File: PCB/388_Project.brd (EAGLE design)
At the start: 88.6 x 79.1 mm, 37 parts, among them IC1 7824DT, U1 ATMEGA328P_TQFP

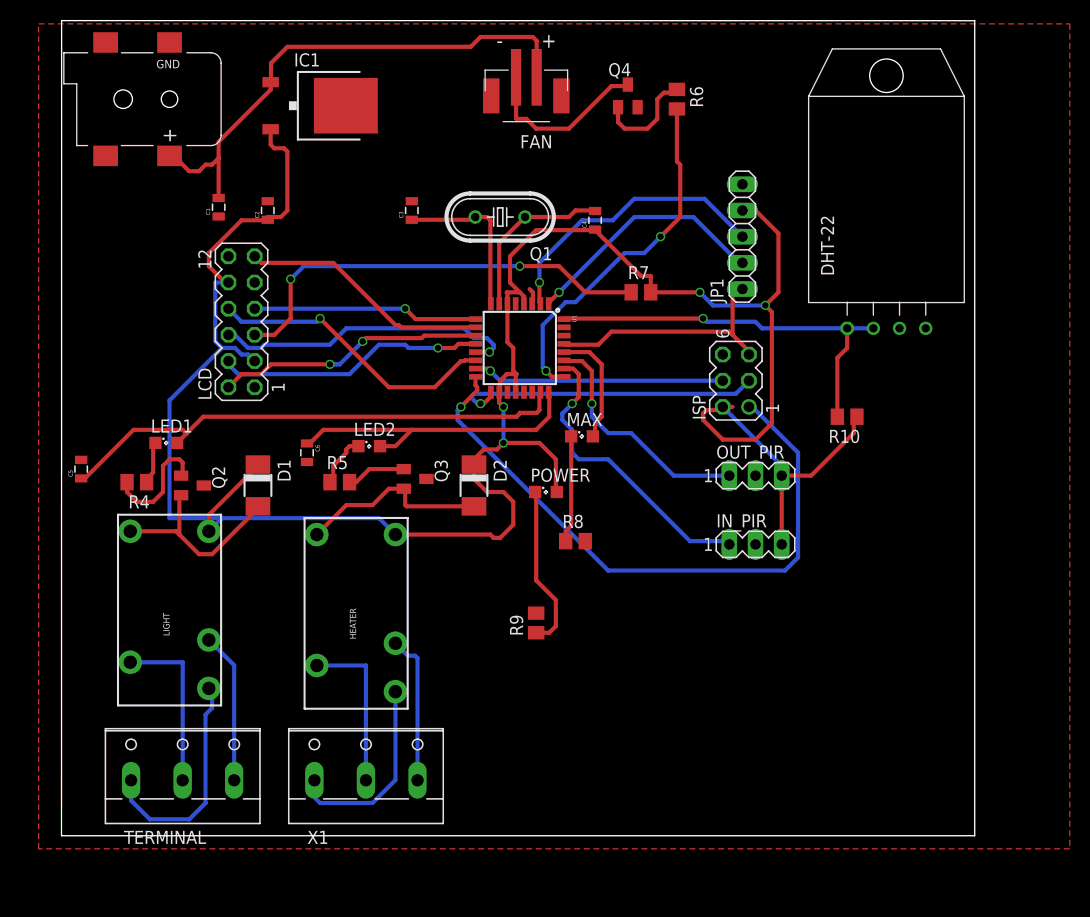
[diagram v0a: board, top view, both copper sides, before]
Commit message: Add files via upload
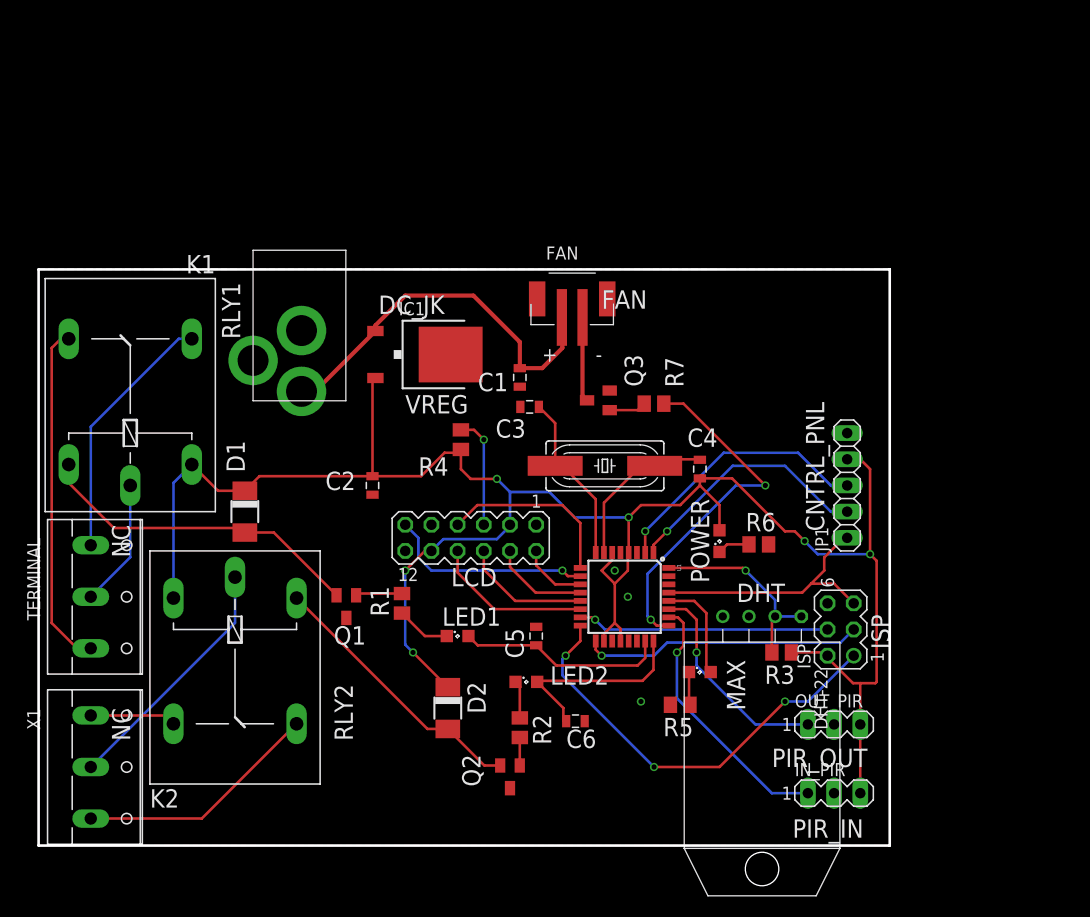
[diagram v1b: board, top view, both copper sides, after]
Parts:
- removed CN1: (no value), adafruit:DCJACK_2MM_SMT
- removed HEATER, LIGHT: RELAYPTH4, SparkFun-Electromechanical:RELAY-JZC
- removed Q4: (no value), adafruit:SOT23
- removed R10: 10k, resistor:M0805
- removed R8, R9: 150, resistor:M0805
- added CRYST: (no value), crystal:HC49UP
- added K1, K2: G5LE, ECE388:G5LE
- added R1, R2: 150, resistor:M0805
- added R3: 10k, resistor:M0805
- added U$1: 2.1MMJACKTHM, ECE388:PJ-102A
- Q1: device crystal:HC49U-V -> semicon-smd-ipc:SOT23
- Q3: device semicon-smd-ipc:SOT23 -> adafruit:SOT23
- R4: value 150 -> 120
- R6: value 10k -> 150
- R7: value 120 -> 10k
- X1: value (none) -> NC
- moved C5 47.0 mm to (48.3, 20.3)
- moved R6 43.9 mm to (69.8, 29.2), turned to 0 degrees
- moved Q2 41.8 mm to (45.7, 6.67), turned to 180 degrees
- moved Q1 40.6 mm to (29.8, 23.2)
- moved R5 39.5 mm to (62.2, 13.7), turned to 180 degrees
- moved C6 36.8 mm to (52.1, 12.1), turned to 0 degrees
- moved LED1 33.9 mm to (40.6, 20.3)
- moved C1 33.6 mm to (46.7, 45.4)
- moved R4 31.7 mm to (41.0, 39.4), turned to 270 degrees
- moved LCD 30.5 mm to (41.9, 29.8), turned to 180 degrees
- moved DHT-22 30.4 mm to (70.2, 22.2), turned to 180 degrees
- moved C2 28.5 mm to (32.4, 34.9), turned to 270 degrees
- moved LED2 27.5 mm to (47.3, 15.9)
- moved ISP 26.2 mm to (77.8, 21.0)
- moved JP1 26.2 mm to (78.4, 34.9)
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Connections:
- net +12V: now also U$1.TIP; no longer CN1.PWR1
- net +5V: now also K1.1, K2.1, R3.1, R4.2; no longer HEATER.5, LIGHT.5, R10.1, R7.2
- net DHT: now also R3.2; no longer R10.2
- net FAN: now also R7.2; no longer R6.2
- net FAN_GND: now also Q3.3; no longer Q4.3
- net GND: now also Q1.3, Q3.2, R5.2, R6.2, U$1.RING, U$1.RING_SW; no longer CN1.GND, CN1.GNDBREAK, Q3.3, Q4.2, R8.2, R9.2
- net N$1: now also K1.O, TERMINAL.3; no longer HEATER.3, X1.1
- net N$10: now also Q2.1, R2.2; no longer Q3.1, R5.2
- net N$11: now also K1.2, Q1.2; no longer LIGHT.1, Q2.2
- net N$12: now also K2.2, Q2.2; no longer HEATER.1, Q3.2
- net N$14: now also R5.1; no longer R8.1
- net N$15: now also R6.1; no longer R9.1
- net N$16: now also K2.O, X1.3; no longer LIGHT.3, TERMINAL.1
- net N$17: now also K2.S, X1.1; no longer LIGHT.4, TERMINAL.2
- net N$18: now also K2.P, X1.2; no longer LIGHT.2, TERMINAL.3
- net N$2: now also Q3.1, R7.1; no longer Q4.1, R6.1
- net N$25: now also R4.1; no longer R7.1
- net N$3: now also CRYST.2; no longer Q1.2
- net N$4: now also CRYST.1; no longer Q1.1
- net N$5: now also K1.S, TERMINAL.1; no longer HEATER.4, X1.2
- net N$6: now also K1.P, TERMINAL.2; no longer HEATER.2, X1.3
- net N$7: now also R1.1; no longer R4.1
- net N$8: now also R2.1; no longer R5.1
- net N$9: now also Q1.1, R1.2; no longer Q2.1, R4.2
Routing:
- net +5V: track 235.4 -> 197.0 mm, vias 4 -> 6
- net N$25: track 42.6 -> 10.9 mm, vias 2 -> 1
- net RELAY_1: track 50.6 -> 20.3 mm
- net DHT: track 39.4 -> 19.4 mm
- net D4: track 26.0 -> 6.44 mm, vias 2 -> 0
- net MISO: track 61.4 -> 42.3 mm, vias 1 -> 3
- net D6: track 29.9 -> 12.4 mm, vias 1 -> 0
- net D5: track 26.2 -> 9.41 mm, vias 1 -> 0
- net +12V: track 52.2 -> 37.7 mm
- net N$1: track 19.2 -> 33.5 mm
- net N$11: track 19.2 -> 32.3 mm
- net D7: track 28.5 -> 15.5 mm, vias 1 -> 0
- net N$15: track 16.1 -> 3.16 mm
- net RELAY_2: track 30.7 -> 19.7 mm
- net N$18: track 14.6 -> 24.2 mm
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- added copper zone on layer 16, net GND
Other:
- board size 88.6 x 79.1 mm -> 82.5 x 55.9 mm
- board text added: "CNTRL_PNL"
- board text added: "DC_JK"
- board text added: "DHT"
- board text added: "FAN"
- board text added: "ISP"
- board text added: "NC"
- board text added: "PIR_IN"
- board text added: "PIR_OUT"
- board text added: "RLY1"
- board text added: "RLY2"
- board text added: "VREG"
